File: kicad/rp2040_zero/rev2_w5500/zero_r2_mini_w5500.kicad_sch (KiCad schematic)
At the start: 6 parts, among them J3 RP2040 Debug, J5 Debug port, Q1 DMG2302U, U1 RP2040-Zero

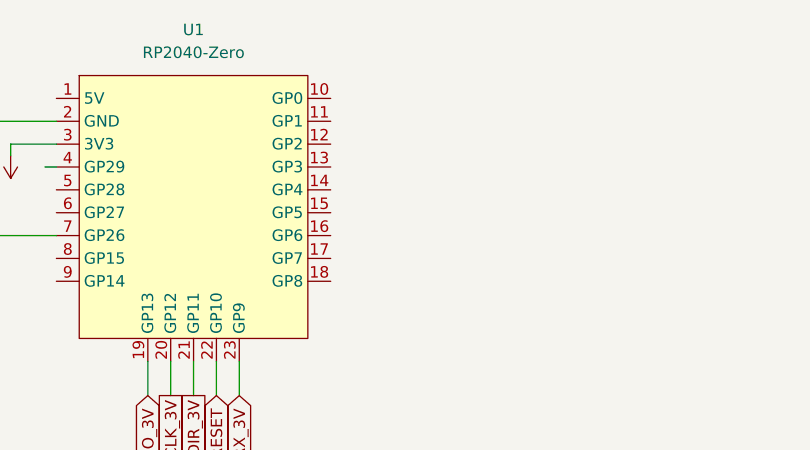
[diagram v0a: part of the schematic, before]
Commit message: w5500 : update 1
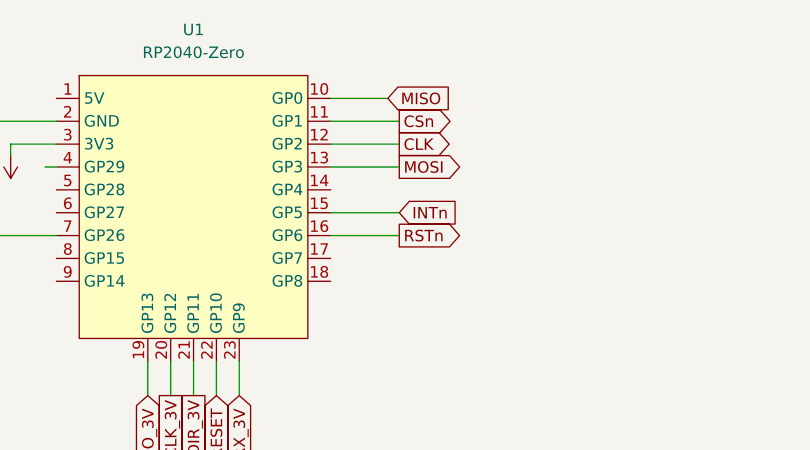
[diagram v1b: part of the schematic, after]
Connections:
- net MISO: now reaches U1.10 (GP0)
- net CSn: now reaches U1.11 (GP1)
- net CLK: now reaches U1.12 (GP2)
- net MOSI: now reaches U1.13 (GP3)
- net INTn: now reaches U1.15 (GP5)
- net RSTn: now reaches U1.16 (GP6)
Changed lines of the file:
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@@
+	(wire
+		(pts
+			(xy 67.31 30.48) (xy 74.93 30.48)
+		)
+		(stroke
+			(width 0)
+			(type default)
+		)
+	)
+	(wire
+		(pts
+			(xy 67.31 22.86) (xy 73.66 22.86)
+		)
+		(stroke
+			(width 0)
+			(type default)
+		)
+	)
 	(wire
 		(pts
@@
 	(wire
 		(pts
+			(xy 67.31 38.1) (xy 74.93 38.1)
+		)
+		(stroke
+			(width 0)
+			(type default)
+		)
+	)
+	(wire
+		(pts
+			(xy 67.31 35.56) (xy 74.93 35.56)
+		)
+		(stroke
+			(width 0)
+			(type default)
+		)
+	)
+	(wire
+		(pts
 			(xy 195.58 40.64) (xy 191.77 40.64)
 		)
@@
 	(wire
 		(pts
+			(xy 67.31 27.94) (xy 74.93 27.94)
+		)
+		(stroke
+			(width 0)
+			(type default)
+		)
+	)
+	(wire
+		(pts
+			(xy 67.31 25.4) (xy 74.93 25.4)
+		)
+		(stroke
+			(width 0)
+			(type default)
+		)
+	)
+	(wire
+		(pts
 			(xy 195.58 43.18) (xy 191.77 43.18)
 		)
@@
 		)
 	)
+	(global_label "MISO"
+		(shape input)
+		(at 73.66 22.86 0)
+		(fields_autoplaced yes)
+		(effects
+			(font
+				(size 1.27 1.27)
+			)
+			(justify left)
+		)
+		(property "Intersheetrefs" "${INTERSHEET_REFS}"
+			(at 81.2414 22.86 0)
+			(hide yes)
+			(show_name no)
+			(do_not_autoplace no)
+			(effects
+				(font
+					(size 1.27 1.27)
+				)
+				(justify left)
+			)
+		)
+	)
 	(global_label "INOUT_NRESET"
 		(shape input)
@@
 				)
 				(justify right)
+			)
+		)
+	)
+	(global_label "RSTn"
+		(shape output)
+		(at 74.93 38.1 0)
+		(fields_autoplaced yes)
+		(effects
+			(font
+				(size 1.27 1.27)
+			)
+			(justify left)
+		)
+		(property "Intersheetrefs" "${INTERSHEET_REFS}"
+			(at 82.5113 38.1 0)
+			(hide yes)
+			(show_name no)
+			(do_not_autoplace no)
+			(effects
+				(font
+					(size 1.27 1.27)
+				)
+				(justify left)
 			)
 		)
@@
 		)
 	)
+	(global_label "INTn"
+		(shape input)
+		(at 74.93 35.56 0)
+		(fields_autoplaced yes)
+		(effects
+			(font
+				(size 1.27 1.27)
+			)
+			(justify left)
+		)
+		(property "Intersheetrefs" "${INTERSHEET_REFS}"
+			(at 81.9671 35.56 0)
+			(hide yes)
+			(show_name no)
+			(do_not_autoplace no)
+			(effects
+				(font
+					(size 1.27 1.27)
+				)
+				(justify left)
+			)
+		)
+	)
 	(global_label "SWDIO"
 		(shape input)
@@
 		)
 	)
+	(global_label "CSn"
+		(shape output)
+		(at 74.93 25.4 0)
+		(fields_autoplaced yes)
+		(effects
+			(font
+				(size 1.27 1.27)
+			)
+			(justify left)
+		)
+		(property "Intersheetrefs" "${INTERSHEET_REFS}"
+			(at 81.5437 25.4 0)
+			(hide yes)
+			(show_name no)
+			(do_not_autoplace no)
+			(effects
+				(font
+					(size 1.27 1.27)
+				)
+				(justify left)
+			)
+		)
+	)
 	(global_label "DRIVE_RESET"
 		(shape input)
@@
 				)
 				(justify right)
+			)
+		)
+	)
+	(global_label "MOSI"
+		(shape output)
+		(at 74.93 30.48 0)
+		(fields_autoplaced yes)
+		(effects
+			(font
+				(size 1.27 1.27)
+			)
+			(justify left)
+		)
+		(property "Intersheetrefs" "${INTERSHEET_REFS}"
+			(at 82.5114 30.48 0)
+			(hide yes)
+			(show_name no)
+			(do_not_autoplace no)
+			(effects
+				(font
+					(size 1.27 1.27)
+				)
+				(justify left)
 			)
 		)
@@
 			(hide yes)
 			(show_name no)
+			(do_not_autoplace no)
+			(effects
+				(font
+					(size 1.27 1.27)
+				)
+				(justify left)
+			)
+		)
+	)
+	(global_label "CLK"
+		(shape output)
+		(at 74.93 27.94 0)
+		(fields_autoplaced yes)
+		(effects
+			(font
+				(size 1.27 1.27)
+			)
+			(justify left)
+		)
+		(property "Intersheetrefs" "${INTERSHEET_REFS}"
+			(at 81.4833 27.94 0)
+			(hide yes)
+			(show_name no)
